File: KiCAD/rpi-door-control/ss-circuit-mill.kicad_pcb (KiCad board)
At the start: 2 copper layers, 103.5 x 49.5 mm, 26 parts, among them IC1 4N35, J1 RJ45, P1 CONN_13X2, P2 CONN_2, P3 CONN_2, P4 CONN_2, Q1 2N3904, Q2 2N3904, SW1 SW_PUSH, U1 RELAY

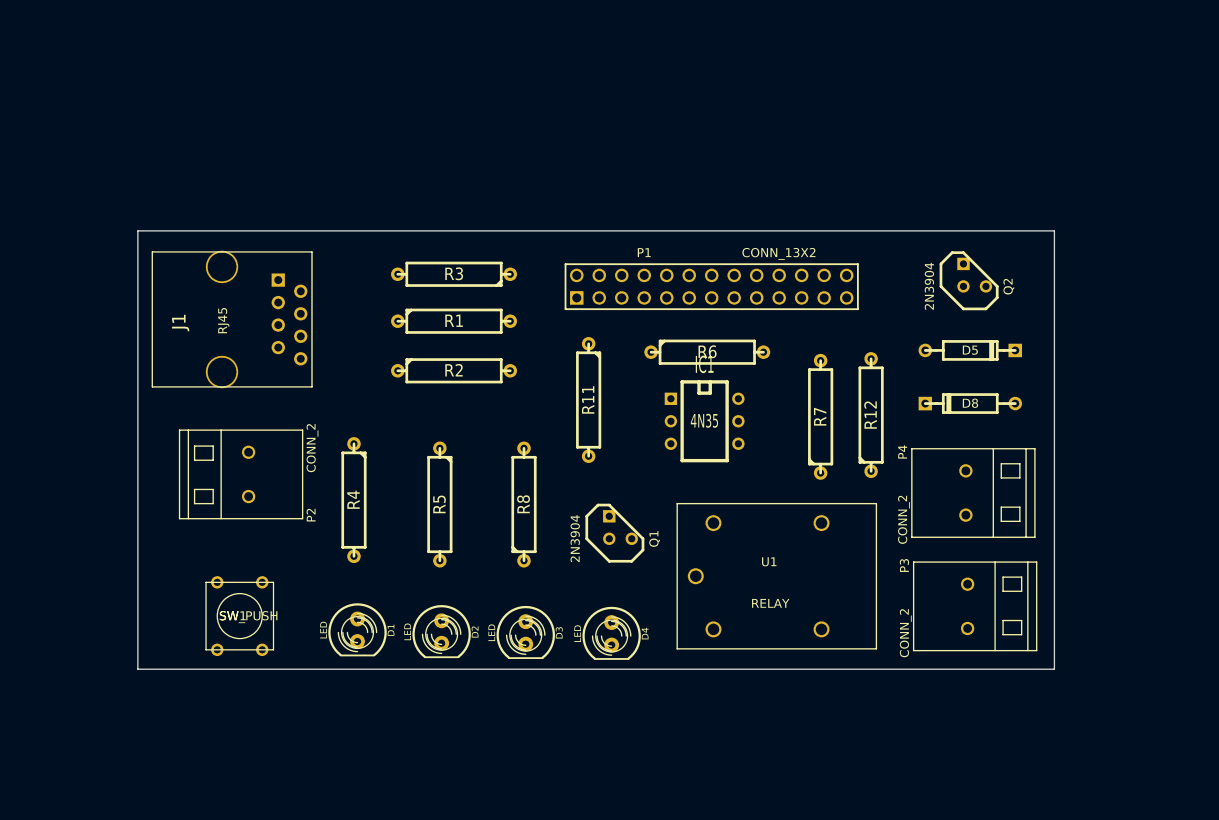
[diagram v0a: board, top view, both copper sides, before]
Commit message: 12V circuit is done but man the data side is tricky
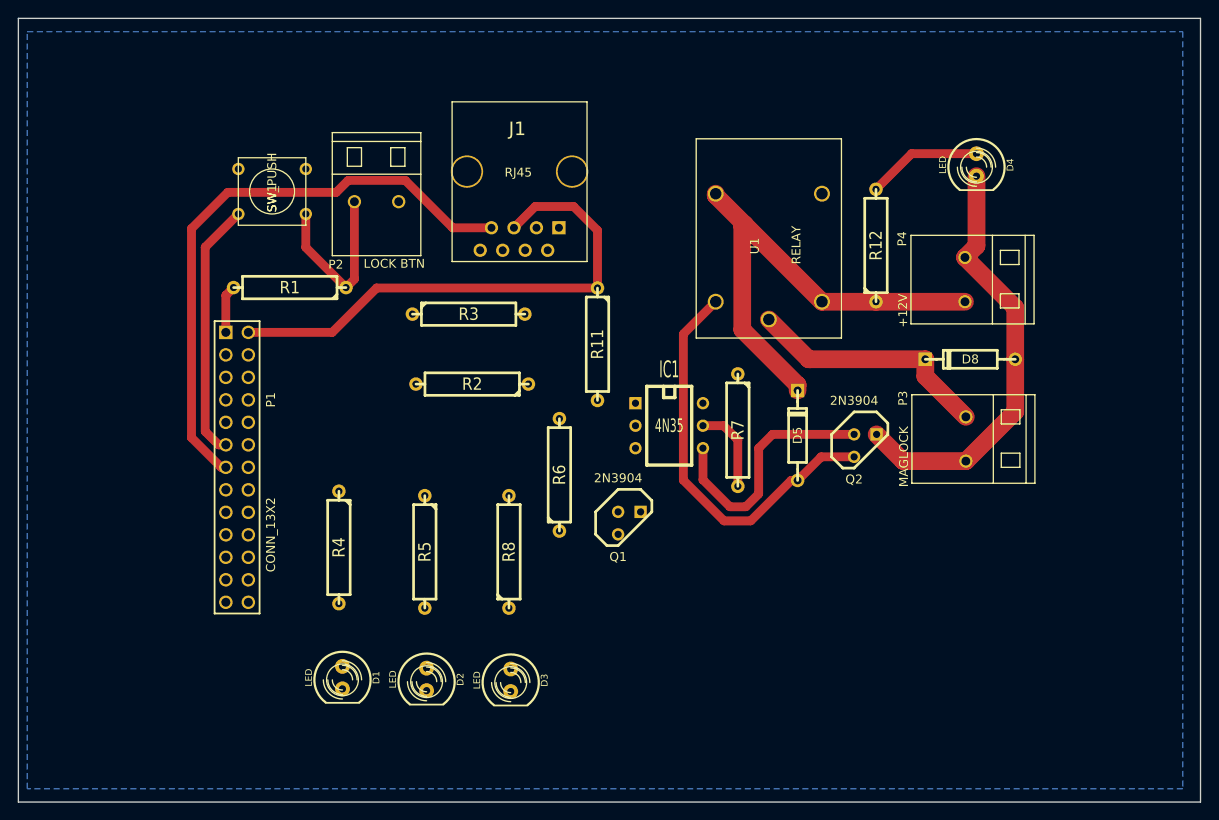
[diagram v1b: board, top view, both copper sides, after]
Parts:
- P2: value CONN_2 -> LOCK BTN
- P3: value CONN_2 -> MAGLOCK
- P4: value CONN_2 -> +12V
- moved D4 67.1 mm to (179.7, 69.5)
- moved P1 57.4 mm to (96.2, 103.7), turned to 270 degrees
- moved SW1 48.1 mm to (100.2, 72.5), turned to 180 degrees
- moved J1 37.5 mm to (128.1, 70.3), turned to 180 degrees
- moved P2 34.0 mm to (112.0, 73.7), turned to 0 degrees
- moved U1 31.6 mm to (156.2, 85.0), turned to 90 degrees
- moved P4 24.1 mm to (178.4, 82.5)
- moved Q2 22.9 mm to (167.2, 101.2), turned to 0 degrees
- moved D5 21.7 mm to (159.5, 100.1), turned to 90 degrees
- moved R6 21.7 mm to (132.6, 104.5), turned to 90 degrees
- moved R12 19.2 mm to (168.3, 78.7)
- moved R1 18.9 mm to (102.2, 83.4), turned to 180 degrees
- moved P3 18.9 mm to (178.5, 100.5)
- moved R7 9.47 mm to (152.8, 99.5), turned to 270 degrees
- moved R11 6.38 mm to (136.9, 89.8)
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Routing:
- net /BELL: track 0.00 -> 67.2 mm
- net +5V: track 0.00 -> 59.6 mm
- net +12V: track 0.00 -> 54.8 mm
- net /GPIO17: track 0.00 -> 49.3 mm
- net GNDPWR: track 0.00 -> 48.7 mm
- net N-0000037: track 0.00 -> 45.8 mm
- net N-0000021: track 0.00 -> 28.3 mm
- net N-0000026: track 0.00 -> 27.9 mm
- net N-0000022: track 0.00 -> 13.0 mm
- net N-000006: track 0.00 -> 9.85 mm
- net +3.3V: track 0.00 -> 5.42 mm
- added copper zone on B.Cu, net (none)
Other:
- board size 103.5 x 49.5 mm -> 133.5 x 88.5 mm
- net class 12V POWER: clearance 2 -> 0.5; trace_width 3 -> 2
- net class Default: clearance 1 -> 0.5
- rule trace_clearance: 1 -> 0.5
